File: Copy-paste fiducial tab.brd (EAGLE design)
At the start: 6.3 x 72.4 mm, 1 part

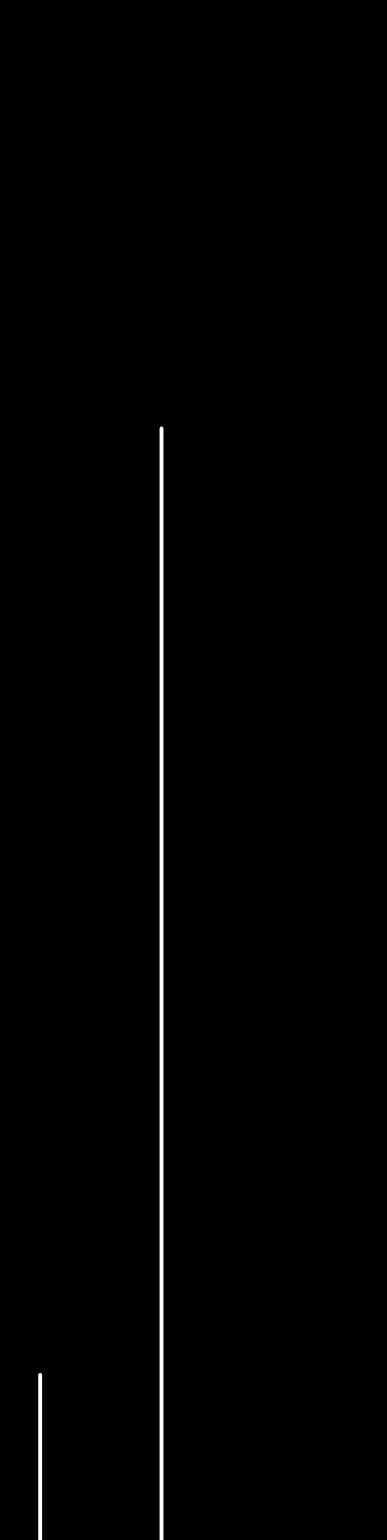
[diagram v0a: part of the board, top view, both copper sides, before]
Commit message: filled out full tab
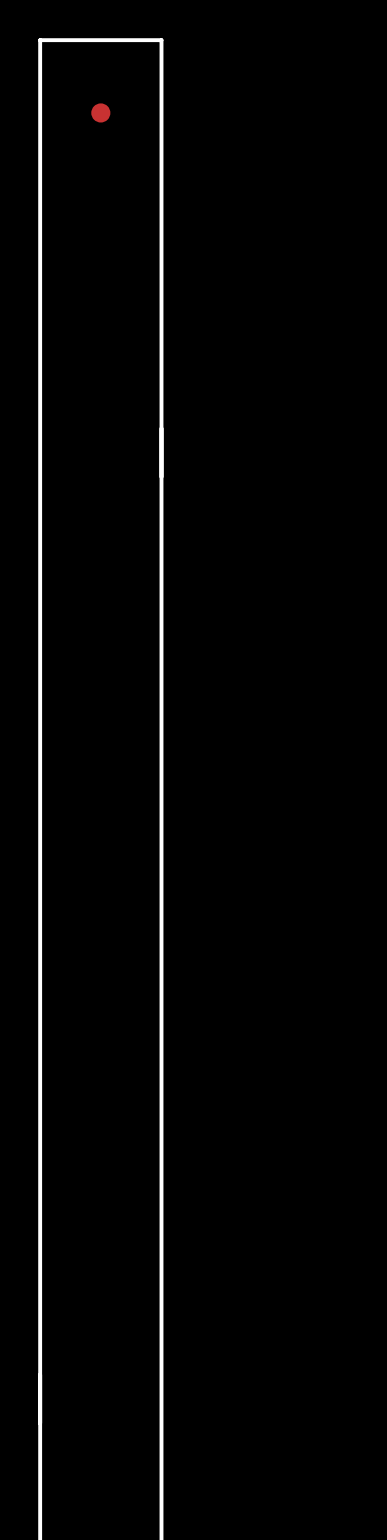
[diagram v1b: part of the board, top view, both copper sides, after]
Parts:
- added E$2: (no value), SparkFun-Aesthetics:FIDUCIAL-1X2
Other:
- board size 6.3 x 72.4 mm -> 6.3 x 92.7 mm
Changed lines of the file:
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@@
 <?xml version="1.0" encoding="utf-8"?>
 <!DOCTYPE eagle SYSTEM "eagle.dtd">
-<eagle version="6.5.0">
+<eagle version="7.3.0">
 <drawing>
 <settings>
@@
 <text x="39.37" y="48.26" size="2.1844" layer="27" font="vector" ratio="12">Copy and paste into panel for fiducial tabs</text>
 <text x="38.1" y="39.37" size="2.54" layer="20" font="vector" ratio="7">Updated 10-30-13. Wider tab</text>
+<wire x1="0" y1="92.71" x2="0" y2="20.32" width="0.2032" layer="20"/>
+<wire x1="6.35" y1="92.71" x2="0" y2="92.71" width="0.2032" layer="20"/>
+<wire x1="6.35" y1="92.71" x2="6.35" y2="69.85" width="0.2032" layer="20"/>
 </plain>
 <attributes>
@@
 <pass name="Default">
 <param name="RoutingGrid" value="50mil"/>
+<param name="AutoGrid" value="1"/>
+<param name="Efforts" value="0"/>
+<param name="TopRouterVariant" value="1"/>
 <param name="tpViaShape" value="round"/>
 <param name="PrefDir.1" value="|"/>
@@
 <elements>
 <element name="E$1" library="SparkFun-Aesthetics" package="FIDUCIAL-1X2" value="" x="3.175" y="3.81"/>
+<element name="E$2" library="SparkFun-Aesthetics" package="FIDUCIAL-1X2" value="" x="3.175" y="88.9" rot="R180"/>
 </elements>
 <signals>
